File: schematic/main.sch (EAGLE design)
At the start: 38 parts, among them IC1 FT232RL, U1 SI4463-C2A-GM, U2 CG2179M2, U3 STM32L011, X1 SMA

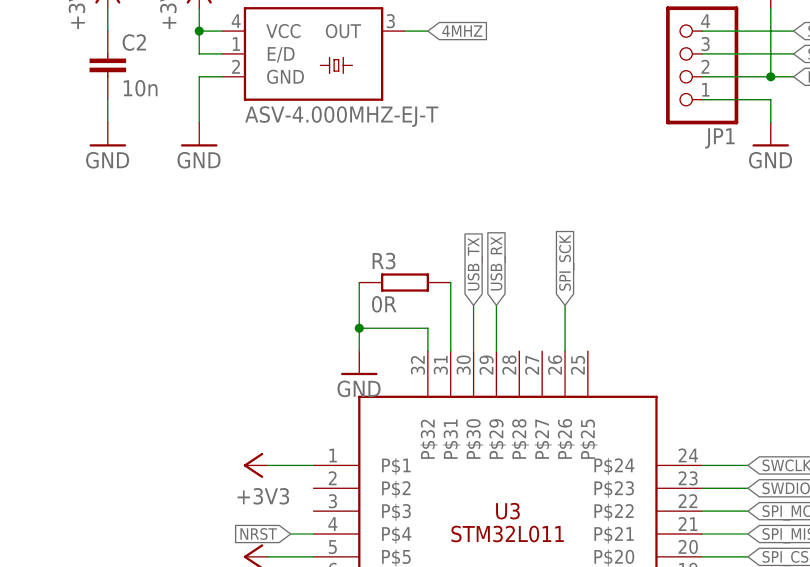
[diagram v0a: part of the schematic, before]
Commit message: Add files via upload
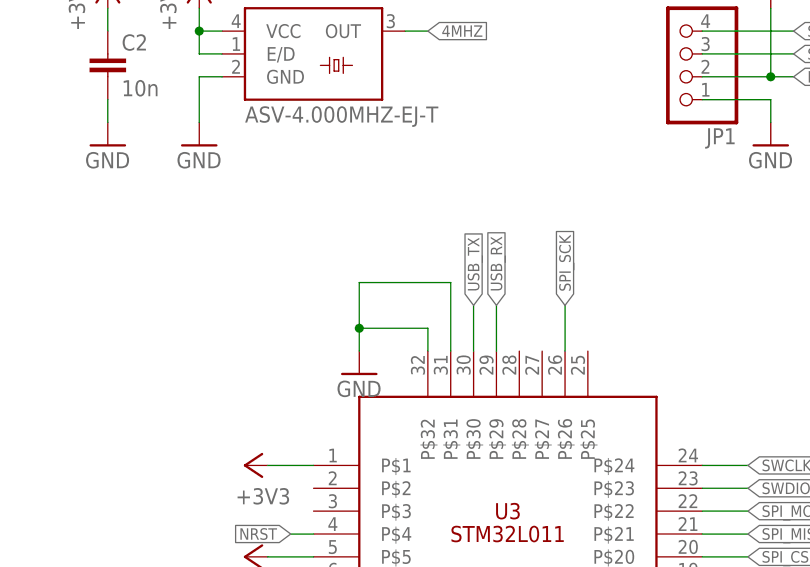
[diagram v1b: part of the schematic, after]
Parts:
- removed R3: 0R, resistor:R-EU_R0805
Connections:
- removed net N$1: R3.2, U3.P$31
- net GND: now also U3.P$31; no longer R3.1
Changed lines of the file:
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@@
 <part name="+3V7" library="supply1" deviceset="+3V3" device=""/>
 <part name="GND9" library="supply1" deviceset="GND" device=""/>
-<part name="R3" library="resistor" deviceset="R-EU_" device="R0805" value="0R"/>
 <part name="QG1" library="crystal" deviceset="SM77H" device="" value="ASV-4.000MHZ-EJ-T"/>
 <part name="+3V6" library="supply1" deviceset="+3V3" device=""/>
@@
 <instance part="+3V7" gate="G$1" x="149.86" y="60.96" rot="R90"/>
 <instance part="GND9" gate="1" x="162.56" y="71.12"/>
-<instance part="R3" gate="G$1" x="167.64" y="81.28"/>
 <instance part="QG1" gate="G$1" x="157.48" y="106.68"/>
 <instance part="+3V6" gate="G$1" x="144.78" y="114.3"/>
@@
 <wire x1="162.56" y1="76.2" x2="170.18" y2="76.2" width="0.1524" layer="91"/>
 <wire x1="170.18" y1="76.2" x2="170.18" y2="73.66" width="0.1524" layer="91"/>
-<pinref part="R3" gate="G$1" pin="1"/>
 <wire x1="162.56" y1="81.28" x2="162.56" y2="76.2" width="0.1524" layer="91"/>
 <junction x="162.56" y="76.2"/>
+<pinref part="U3" gate="G$1" pin="P$31"/>
+<wire x1="172.72" y1="81.28" x2="172.72" y2="73.66" width="0.1524" layer="91"/>
+<wire x1="162.56" y1="81.28" x2="172.72" y2="81.28" width="0.1524" layer="91"/>
 </segment>
 <segment>
@@
 </segment>
 </net>
-<net name="N$1" class="0">
-<segment>
-<pinref part="R3" gate="G$1" pin="2"/>
-<pinref part="U3" gate="G$1" pin="P$31"/>
-<wire x1="172.72" y1="81.28" x2="172.72" y2="73.66" width="0.1524" layer="91"/>
-</segment>
-</net>
